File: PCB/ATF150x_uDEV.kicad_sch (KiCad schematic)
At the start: 16 parts, among them J1 Conn_02x05_Odd_Even, J2 VERT, J3 VERT, U1 ATF150x-xAx44

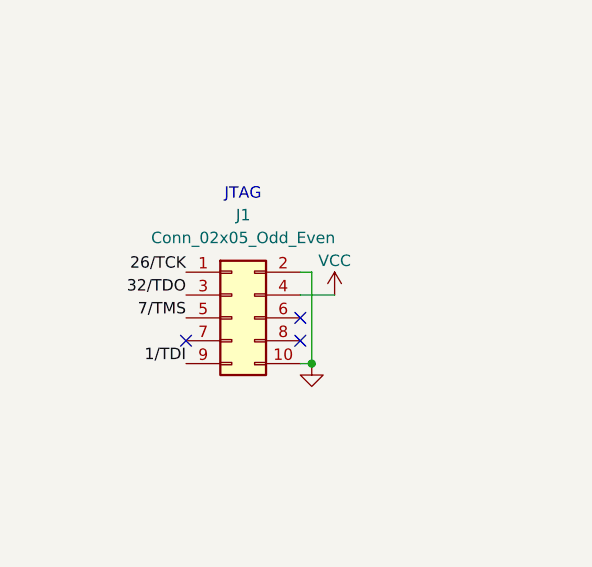
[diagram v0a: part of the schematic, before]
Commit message: jtag symbols
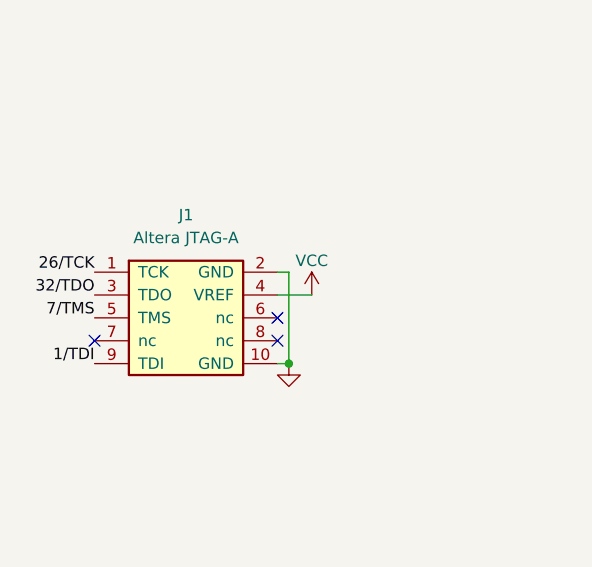
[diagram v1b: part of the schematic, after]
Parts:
- removed J1: Conn_02x05_Odd_Even, 000_LOCAL:IDC-Header_2x05_P2.54mm_Vertical, symbol 000_LOCAL:Conn_02x05_Odd_Even
- added J1: Altera JTAG-A, symbol 000_LOCAL:Altera JTAG-A
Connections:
- net 1/TDI: now also J1.9 (TDI)
- net 26/TCK: now also J1.1 (TCK)
- net 32/TDO: now also J1.3 (TDO)
- net 7/TMS: now also J1.5 (TMS)
- net GND: now also J1.10 (GND), J1.2 (GND)
- net VCC: now also J1.4 (VREF)
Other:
- note removed: "JTAG"
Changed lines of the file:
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@@
 	)
 	(junction
-		(at 71.12 93.98)
+		(at 68.58 93.98)
 		(diameter 0)
 		(color 0 0 0 0)
 	)
 	(no_connect
-		(at 69.85 91.44)
+		(at 67.31 91.44)
 	)
 	(no_connect
-		(at 57.15 91.44)
+		(at 46.99 91.44)
 	)
 	(no_connect
-		(at 69.85 88.9)
+		(at 67.31 88.9)
 	)
 	(wire
@@
 	(wire
 		(pts
-			(xy 71.12 83.82) (xy 71.12 93.98)
+			(xy 68.58 83.82) (xy 68.58 93.98)
 		)
 		(stroke
@@
 	(wire
 		(pts
-			(xy 73.66 86.36) (xy 69.85 86.36)
+			(xy 71.12 86.36) (xy 67.31 86.36)
 		)
 		(stroke
@@
 	(wire
 		(pts
-			(xy 71.12 93.98) (xy 69.85 93.98)
+			(xy 68.58 93.98) (xy 67.31 93.98)
 		)
 		(stroke
@@
 	(wire
 		(pts
-			(xy 69.85 83.82) (xy 71.12 83.82)
+			(xy 67.31 83.82) (xy 68.58 83.82)
 		)
 		(stroke
@@
 		)
 	)
-	(text "JTAG"
-		(exclude_from_sim no)
-		(at 65.532 75.946 0)
-		(effects
-			(font
-				(size 1.27 1.27)
-			)
-			(justify right bottom)
-		)
-	)
 	(label "13"
 		(at 124.46 93.98 180)
@@
 	)
 	(label "32{slash}TDO"
-		(at 57.15 86.36 180)
+		(at 46.99 86.36 180)
 		(fields_autoplaced yes)
 		(effects
@@
 	)
 	(label "26{slash}TCK"
-		(at 57.15 83.82 180)
+		(at 46.99 83.82 180)
 		(fields_autoplaced yes)
 		(effects
@@
 	)
 	(label "1{slash}TDI"
-		(at 57.15 93.98 180)
+		(at 46.99 93.98 180)
 		(fields_autoplaced yes)
 		(effects
@@
 	)
 	(label "7{slash}TMS"
-		(at 57.15 88.9 180)
+		(at 46.99 88.9 180)
 		(fields_autoplaced yes)
 		(effects
@@
 	(symbol
 		(lib_id "power:VCC")
-		(at 73.66 86.36 0)
+		(at 71.12 86.36 0)
 		(unit 1)
 		(exclude_from_sim no)
@@
 		(dnp no)
 		(property "Reference" "#PWR010"
-			(at 73.66 90.17 0)
+			(at 71.12 90.17 0)
 			(effects
 				(font
@@
 		)
 		(property "Value" "VCC"
-			(at 73.66 82.55 0)
+			(at 71.12 82.55 0)
 			(effects
 				(font
@@
 		)
 		(property "Footprint" ""
-			(at 73.66 86.36 0)
+			(at 71.12 86.36 0)
 			(effects
 				(font
@@
 		)
 		(property "Datasheet" ""
-			(at 73.66 86.36 0)
+			(at 71.12 86.36 0)
 			(effects
 				(font
@@
 		)
 		(property "Description" "Power symbol creates a global label with name \"VCC\""
-			(at 73.66 86.36 0)
+			(at 71.12 86.36 0)
 			(effects
 				(font
@@
 				(path "/59fc349f-54da-4a51-bb89-375ab443b404"
 					(reference "#PWR010")
-					(unit 1)
-				)
-			)
-		)
-	)
-	(symbol
-		(lib_id "000_LOCAL:Conn_02x05_Odd_Even")
-		(at 62.23 88.9 0)
-		(unit 1)
-		(exclude_from_sim no)
-		(in_bom yes)
-		(on_board yes)
-		(dnp no)
-		(fields_autoplaced yes)
-		(property "Reference" "J1"
-			(at 63.5 77.47 0)
-			(effects
-				(font
-					(size 1.27 1.27)
-				)
-			)
-		)
-		(property "Value" "Conn_02x05_Odd_Even"
-			(at 63.5 80.01 0)
-			(effects
-				(font
-					(size 1.27 1.27)
-				)
-			)
-		)
-		(property "Footprint" "000_LOCAL:IDC-Header_2x05_P2.54mm_Vertical"
-			(at 62.23 88.9 0)
-			(effects
-				(font
-					(size 1.27 1.27)
-				)
-				(hide yes)
-			)
-		)
-		(property "Datasheet" "datasheets/JTAG-A.pdf"
-			(at 62.23 88.9 0)
-			(effects
-				(font
-					(size 1.27 1.27)
-				)
-				(hide yes)
-			)
-		)
-		(property "Description" "Generic connector, double row, 02x05, odd/even pin numbering scheme (row 1 odd numbers, row 2 even numbers), script generated (kicad-library-utils/schlib/autogen/connector/)"
-			(at 62.23 88.9 0)
-			(effects
-				(font
-					(size 1.27 1.27)
-				)
-				(hide yes)
-			)
-		)
-		(pin "7"
-		)
-		(pin "6"
-		)
-		(pin "5"
-		)
-		(pin "9"
-		)
-		(pin "8"
-		)
-		(pin "1"
-		)
-		(pin "3"
-		)
-		(pin "10"
-		)
-		(pin "2"
-		)
-		(pin "4"
-		)
-		(instances
-			(project "ATF1502AS_uDEV"
-				(path "/59fc349f-54da-4a51-bb89-375ab443b404"
-					(reference "J1")
 					(unit 1)
 				)
@@
 	(symbol
 		(lib_id "power:GND")
-		(at 71.12 93.98 0)
+		(at 68.58 93.98 0)
 		(unit 1)
 		(exclude_from_sim no)
@@
 		(dnp no)
 		(property "Reference" "#PWR01"
-			(at 71.12 100.33 0)
+			(at 68.58 100.33 0)
 			(effects
 				(font
@@
 		)
 		(property "Value" "GND"
-			(at 71.12 98.298 0)
+			(at 68.58 98.298 0)
 			(effects
 				(font
@@
 		)
 		(property "Footprint" ""
-			(at 71.12 93.98 0)
+			(at 68.58 93.98 0)
 			(effects
 				(font
@@
 		)
 		(property "Datasheet" ""
-			(at 71.12 93.98 0)
+			(at 68.58 93.98 0)
 			(effects
 				(font
@@
 		)
 		(property "Description" "Power symbol creates a global label with name \"GND\" , ground"
-			(at 71.12 93.98 0)
+			(at 68.58 93.98 0)
 			(effects
 				(font
@@
 					(unit 1)
 				)
+			)
+		)
+	)
+	(symbol
+		(lib_id "000_LOCAL:Altera JTAG-A")
+		(at 57.15 88.9 0)
+		(unit 1)
+		(exclude_from_sim no)
+		(in_bom yes)
+		(on_board yes)
+		(dnp no)
+		(fields_autoplaced yes)
+		(property "Reference" "J1"
+			(at 57.15 77.47 0)
+			(effects
+				(font
+					(size 1.27 1.27)
+				)
+			)
+		)
+		(property "Value" "Altera JTAG-A"
+			(at 57.15 80.01 0)
+			(effects
+				(font
+					(size 1.27 1.27)
+				)
+			)
+		)
+		(property "Footprint" ""
+			(at 57.15 88.9 0)
+			(effects
+				(font
+					(size 1.27 1.27)
+				)
+				(hide yes)
+			)
+		)
+		(property "Datasheet" "datasheets/JTAG-A.pdf"
+			(at 57.15 88.9 0)
+			(effects
+				(font
+					(size 1.27 1.27)
+				)
+				(hide yes)
+			)
+		)
+		(property "Description" "Generic connector, double row, 02x05, odd/even pin numbering scheme (row 1 odd numbers, row 2 even numbers), script generated (kicad-library-utils/schlib/autogen/connector/)"
+			(at 57.15 88.9 0)
+			(effects
+				(font
+					(size 1.27 1.27)
+				)
+				(hide yes)
+			)
+		)
+		(pin "4"
+		)
+		(pin "7"
+		)
+		(pin "9"
+		)
+		(pin "8"
+		)
+		(pin "2"
+		)
+		(pin "6"
+		)
+		(pin "10"
+		)
+		(pin "1"
+		)
+		(pin "5"
+		)
+		(pin "3"
+		)
+		(instances
+			(project ""
+				(path "/59fc349f-54da-4a51-bb89-375ab443b404"
+					(reference "J1")
+					(unit 1)
+				)
